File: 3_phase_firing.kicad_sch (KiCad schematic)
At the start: 66 parts, among them J1 IN1, J2 IN2, J3 OUT, J4 USB_B, J5 Conn_01x03, J6 Conn_01x02, J7 Conn_01x03, J8 Conn_01x02, Q1 MMBT3904, Q2 MMBT3904, Q3 MMBT3904, Q4 MMBT3904, Q5 MMBT3904, Q6 MMBT3904, U1 LM339, U10 4N35, U11 4N35, U12 4N35, U2 L7812, U3 4N35, U4 4N35, U5 4N35, U6 YAAJ_WeAct_BlackPill_Part_Like, U7 4N35, U8 4N35, U9 4N35

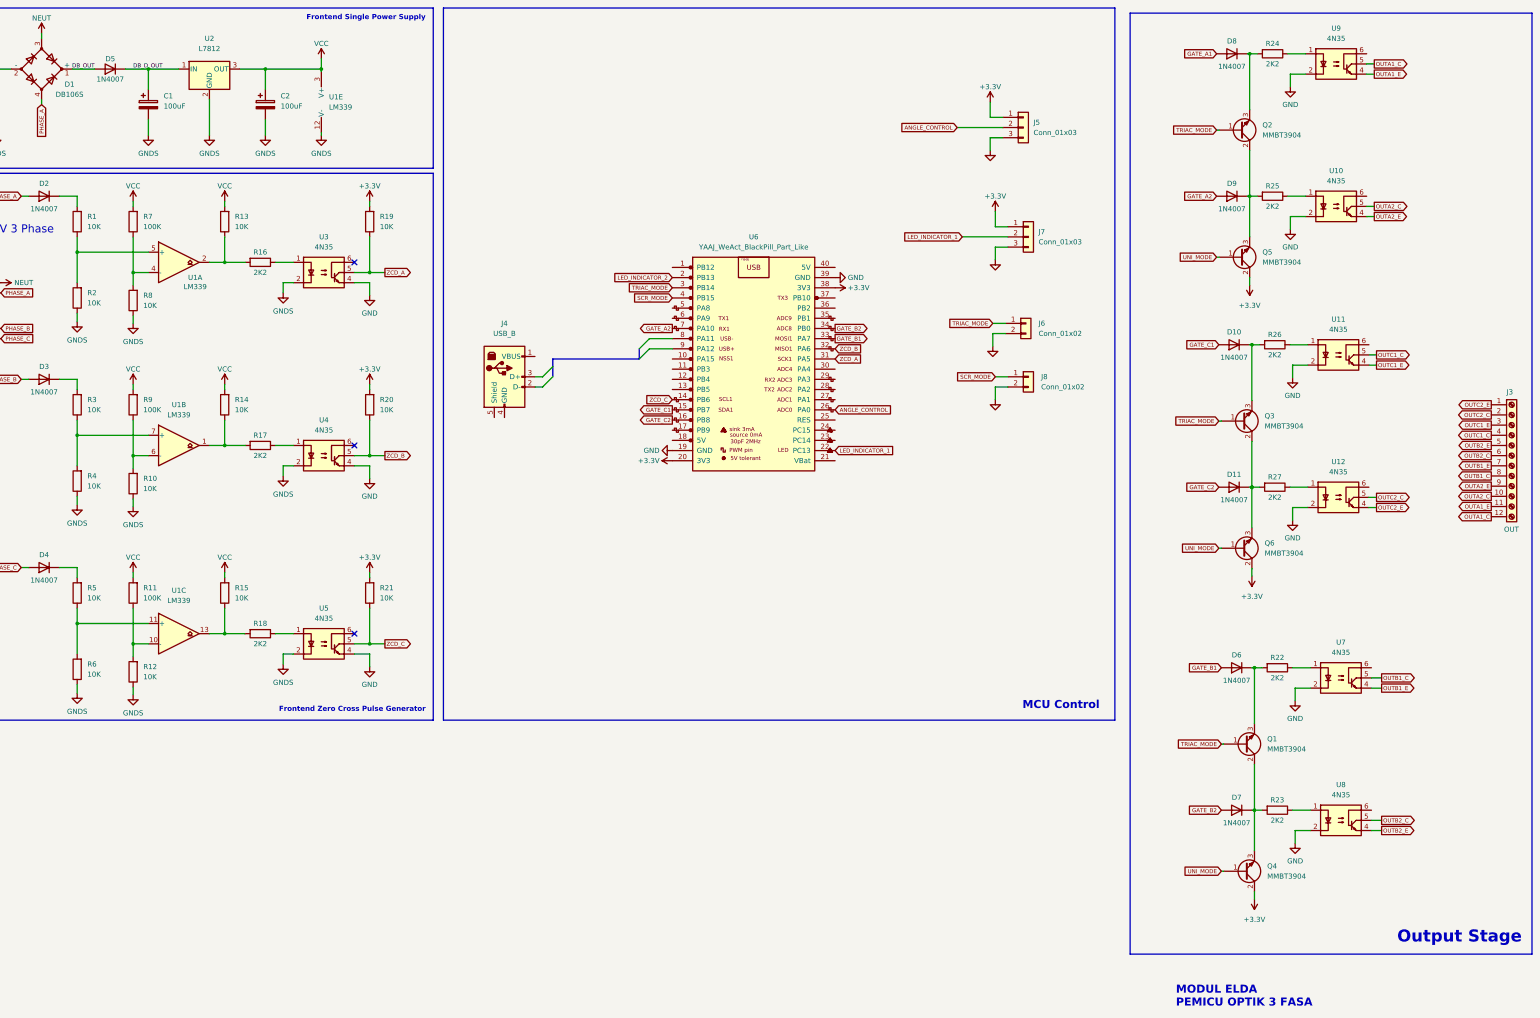
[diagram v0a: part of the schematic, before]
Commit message: done with all revision
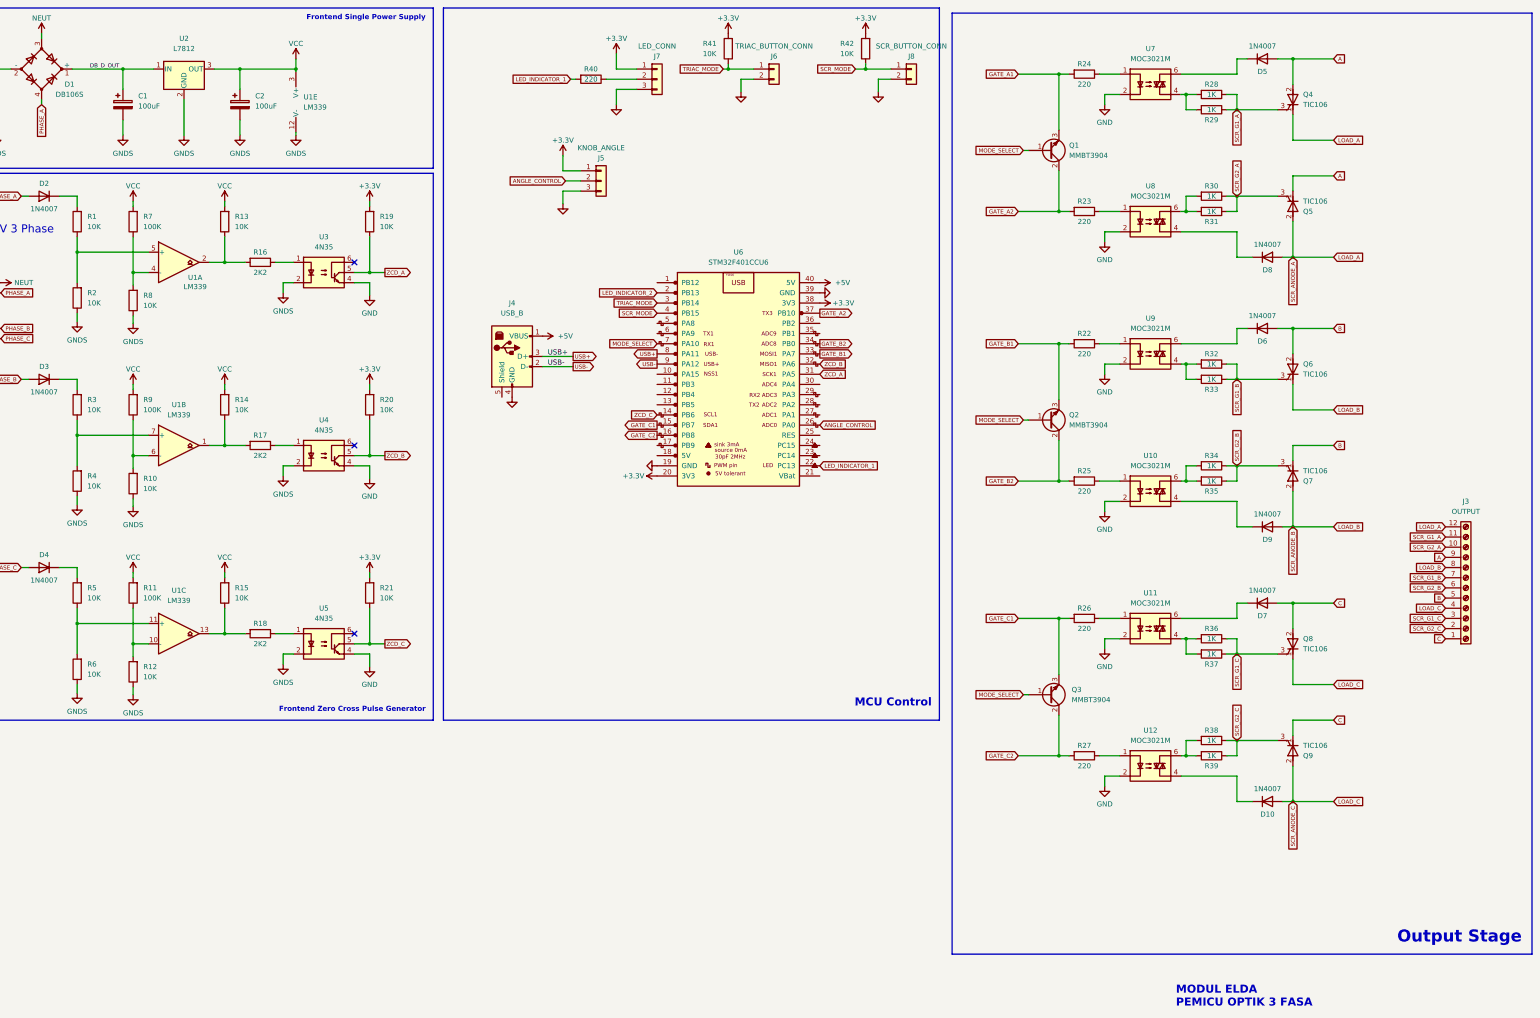
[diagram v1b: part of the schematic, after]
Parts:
- removed D11: 1N4007, Diode_SMD:D_SMA_Handsoldering, symbol Device:D
- removed Q1, Q4, Q5, Q6: MMBT3904, Package_TO_SOT_SMD:SOT-23, symbol Device:Q_NPN_BCE
- removed U10, U11, U12, U7, U8, U9: 4N35, Package_DIP:DIP-6_W8.89mm_SMDSocket_LongPads, symbol Isolator:4N35
- added Q2: MMBT3904, Package_TO_SOT_SMD:SOT-23, symbol Device:Q_NPN_BCE
- added Q4, Q5, Q6, Q7, Q8, Q9: TIC106, Package_TO_SOT_THT:TO-220-3_Vertical, symbol Triac_Thyristor:TIC106
- added R28, R29, R30, R31, R32, R33, R34, R35, R36, R37, R38, R39: 1K, Resistor_SMD:R_1206_3216Metric_Pad1.30x1.75mm_HandSolder, symbol Device:R
- added R40: 220, Resistor_SMD:R_1206_3216Metric_Pad1.30x1.75mm_HandSolder, symbol Device:R
- added R41, R42: 10K, Resistor_SMD:R_0805_2012Metric, symbol Device:R
- added U10, U11, U12, U7, U8, U9: MOC3021M, Package_DIP:DIP-6_W8.89mm_SMDSocket_LongPads, symbol Relay_SolidState:MOC3021M
- J3: value OUT -> OUTPUT; footprint TerminalBlock_Phoenix:TerminalBlock_Phoenix_MKDS-3-12-5.08_1x12_P5.08mm_Horizontal -> TerminalBlock_Phoenix:TerminalBlock_Phoenix_MKDS-1,5-12-5.08_1x12_P5.08mm_Horizontal
- J5: value Conn_01x03 -> KNOB_ANGLE
- J6: value Conn_01x02 -> TRIAC_BUTTON_CONN
- J7: value Conn_01x03 -> LED_CONN
- J8: value Conn_01x02 -> SCR_BUTTON_CONN
- R22, R23, R24, R25, R26, R27: value 2K2 -> 220
- U6: value YAAJ_WeAct_BlackPill_Part_Like -> STM32F401CCU6
- renumbered Q2 to Q1
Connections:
- net OUTA2_E is gone; now on net A: J3.9 (Pin_9)
- net +3.3V: now also R41.2, R42.2
- net DB_D_OUT: now also D1.1 (+); no longer D5.1 (K)
- net GATE_A1: now also Q1.3 (E), R24.2; no longer D8.2 (A)
- net GATE_A2: now also Q1.2 (C), R23.2, U6.37 (PB10); no longer D9.2 (A), U6.7 (PA10)
- net GATE_B1: now also R22.2, Q2.3 (E); no longer D6.2 (A)
- net GATE_B2: now also R25.2, Q2.2 (C); no longer D7.2 (A)
- net GATE_C1: now also Q3.3 (E), R26.2; no longer D10.2 (A)
- net GATE_C2: now also Q3.2 (C), R27.2
- net GND: now also J4.4 (GND), U10.2, U11.2, U12.2, U7.2, U8.2, U9.2
- net LED_INDICATOR_1: now also R40.2; no longer J7.2 (Pin_2)
- net SCR_MODE: now also R42.1
- net TRIAC_MODE: now also R41.1; no longer Q1.1 (B), Q3.1 (B)
- net +5V: now reaches U6.40 (5V)
- net +5V: now also J4.1 (VBUS)
- net USB+: now reaches U6.8 (PA11)
- net USB+: now also J4.3 (D+)
- net USB-: now reaches U6.9 (PA12)
- net USB-: now also J4.2 (D-)
- net at D7.1 (K): now also U11.6; no longer R23.2
- net at R24.1: now also U7.1
- net at R25.1: now also U10.1
- net at R22.1: now also U9.1
- net at R26.1: now also U11.1
- net at R27.1: now also U12.1
- net at R23.1: now also U8.1
- net at D6.1 (K): now also U9.6; no longer R22.2
- net DB_OUT renamed A
- net A: now also Q4.2 (A), Q5.1 (K); no longer D1.1 (+)
- net OUTA1_C renamed LOAD_A
- net LOAD_A: now also D8.2 (A), Q4.1 (K), Q5.2 (A)
- net OUTA1_E renamed SCR_G1_A
- net SCR_G1_A: now also Q4.3 (G), R28.1, R29.1
- net OUTA2_C renamed SCR_G2_A
- net SCR_G2_A: now also Q5.3 (G), R30.1, R31.1
- net OUTB1_C renamed LOAD_B
- net LOAD_B: now also D9.2 (A), Q6.1 (K), Q7.2 (A)
- net OUTB1_E renamed SCR_G1_B
- net SCR_G1_B: now also Q6.3 (G), R32.1, R33.1
- net OUTB2_C renamed SCR_G2_B
- net SCR_G2_B: now also Q7.3 (G), R34.1, R35.1
- net OUTB2_E renamed B
- net B: now also D6.2 (A), Q6.2 (A), Q7.1 (K)
- net OUTC1_C renamed LOAD_C
- net LOAD_C: now also D10.2 (A), Q8.1 (K), Q9.2 (A)
- net OUTC1_E renamed SCR_G1_C
- net SCR_G1_C: now also Q8.3 (G), R36.1, R37.1
- net OUTC2_C renamed SCR_G2_C
- net SCR_G2_C: now also Q9.3 (G), R38.1, R39.1
- net OUTC2_E renamed C
- net C: now also D7.2 (A), Q8.2 (A), Q9.1 (K)
- new net: J7.2 (Pin_2), R40.1
- new net: R28.2, R29.2, U7.4
- new net: D5.1 (K), U7.6
- new net: D9.1 (K), U10.4
- new net: R34.2, R35.2, U10.6
- new net: R32.2, R33.2, U9.4
- new net: R36.2, R37.2, U11.4
- new net: R38.2, R39.2, U12.6
- new net: R30.2, R31.2, U8.6
- new net: D10.1 (K), U12.4
- new net: D8.1 (K), U8.4
- new net MODE_SELECT: Q1.1 (B), Q2.1 (B), Q3.1 (B), U6.7 (PA10)
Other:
- moved on the sheet: C1, C2, J4, J5, J6, J7, J8, Q1, R24, U1E, U2, U6
